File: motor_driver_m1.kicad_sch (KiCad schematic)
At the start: 51 parts, among them J1 Conn_01x01_Pin, J2 Conn_01x01_Pin, J3 Conn_01x01_Pin, M1 STM32C011F6U6TR, Q1 NP80N06D6, Q2 NP80N06D6, Q3 NP80N06D6, Q4 NP80N06D6, Q5 NP80N06D6, Q6 NP80N06D6, U1 STM32G431KBU6

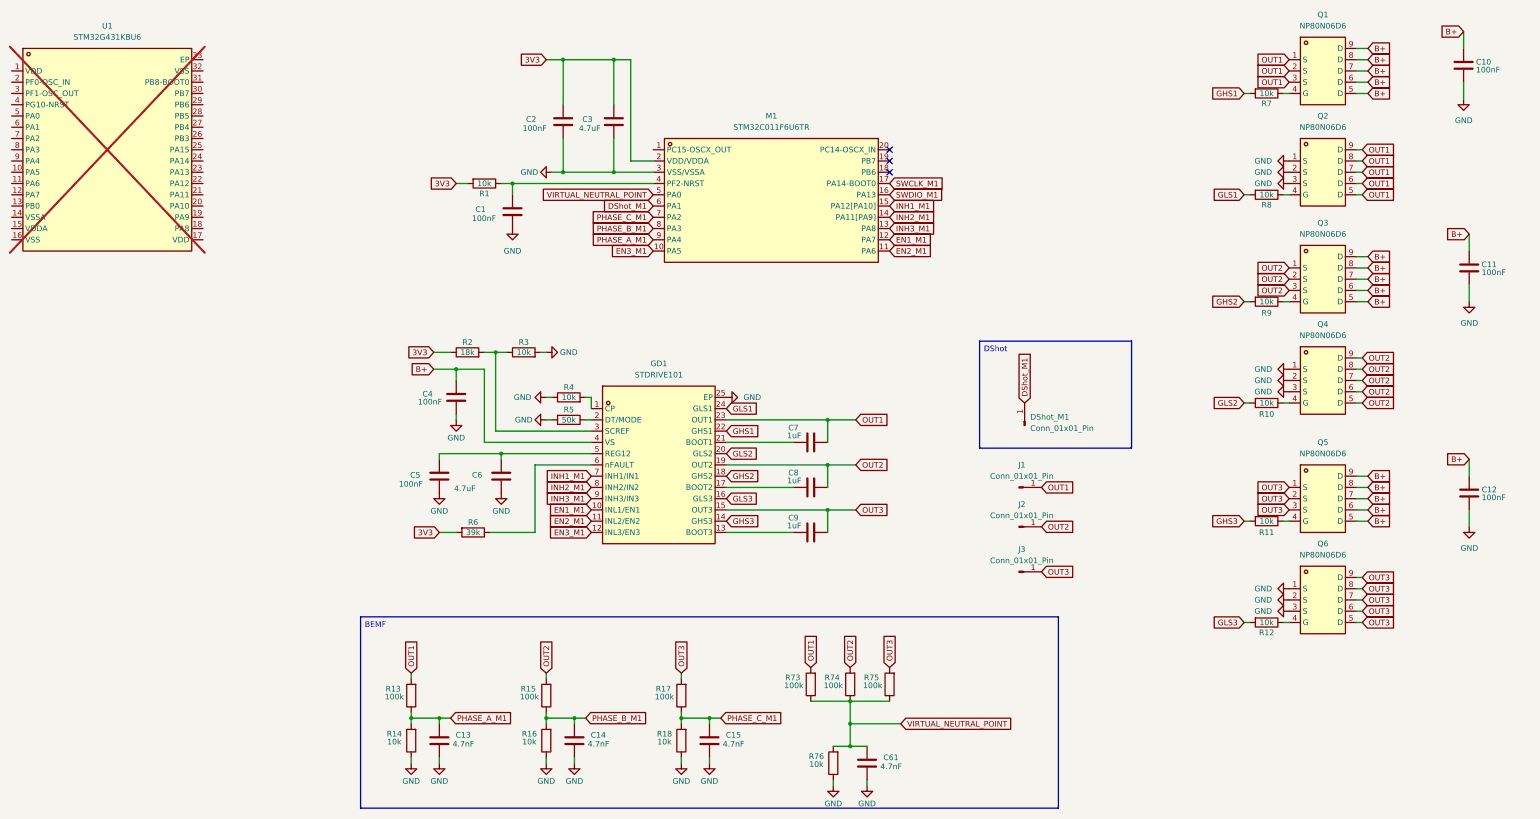
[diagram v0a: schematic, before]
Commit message: ...
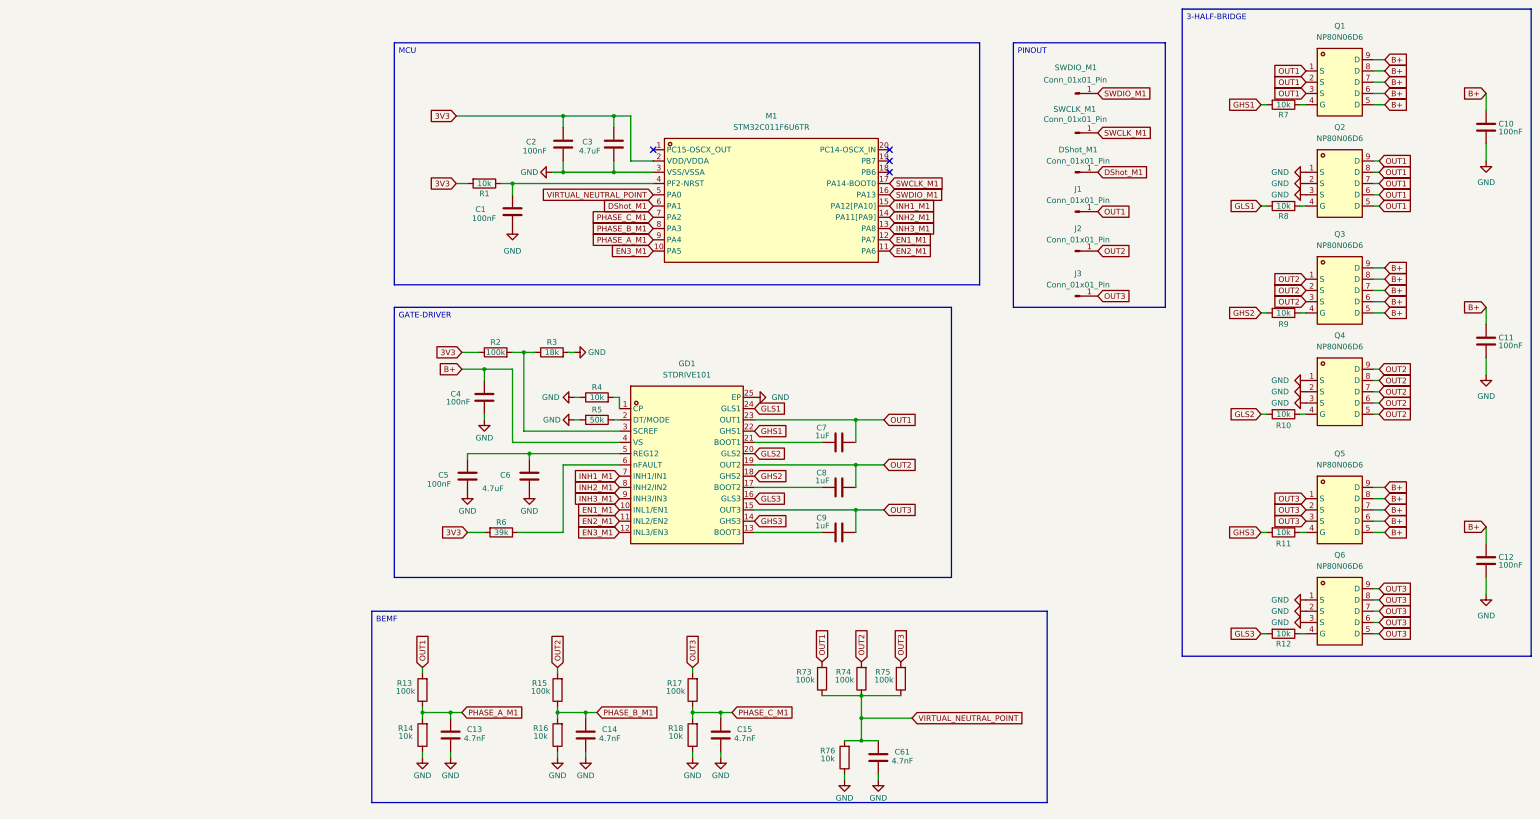
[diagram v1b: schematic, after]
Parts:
- removed U1: STM32G431KBU6, easyeda2kicad:QFN-32_L5.0-W5.0-P0.50-BL-EP3.7, symbol easyeda2kicad:STM32G431KBU6
- added SWCLK_M1, SWDIO_M1: Conn_01x01_Pin, deshan:Conn_01x01_Pin, symbol Connector:Conn_01x01_Pin
- R2: value 18k -> 100k
- R3: value 10k -> 18k
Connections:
- net SWCLK_M1: now also SWCLK_M1.1 (Pin_1)
- net SWDIO_M1: now also SWDIO_M1.1 (Pin_1)
- no-connect marks 3 -> 4
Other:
- moved on the sheet: C10, C11, C12, C13, C14, C15, C2, C3, C4, C5, C6, C61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
